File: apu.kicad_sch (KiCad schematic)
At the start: 0 parts

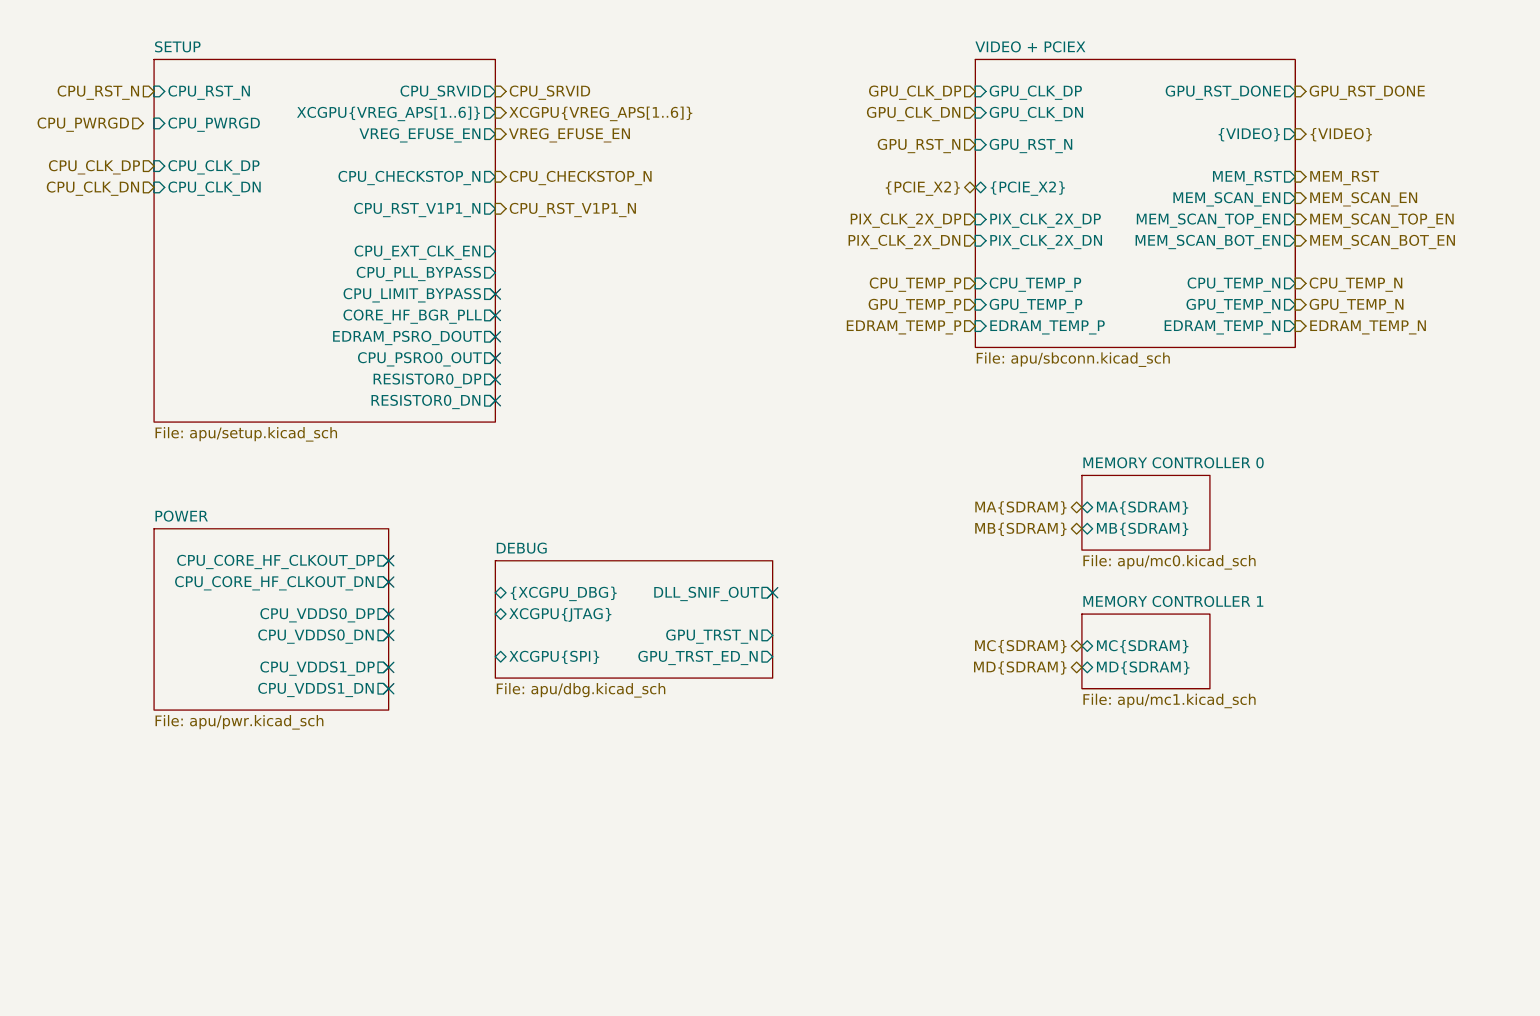
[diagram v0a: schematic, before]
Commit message: Cleanup & Debug I/O
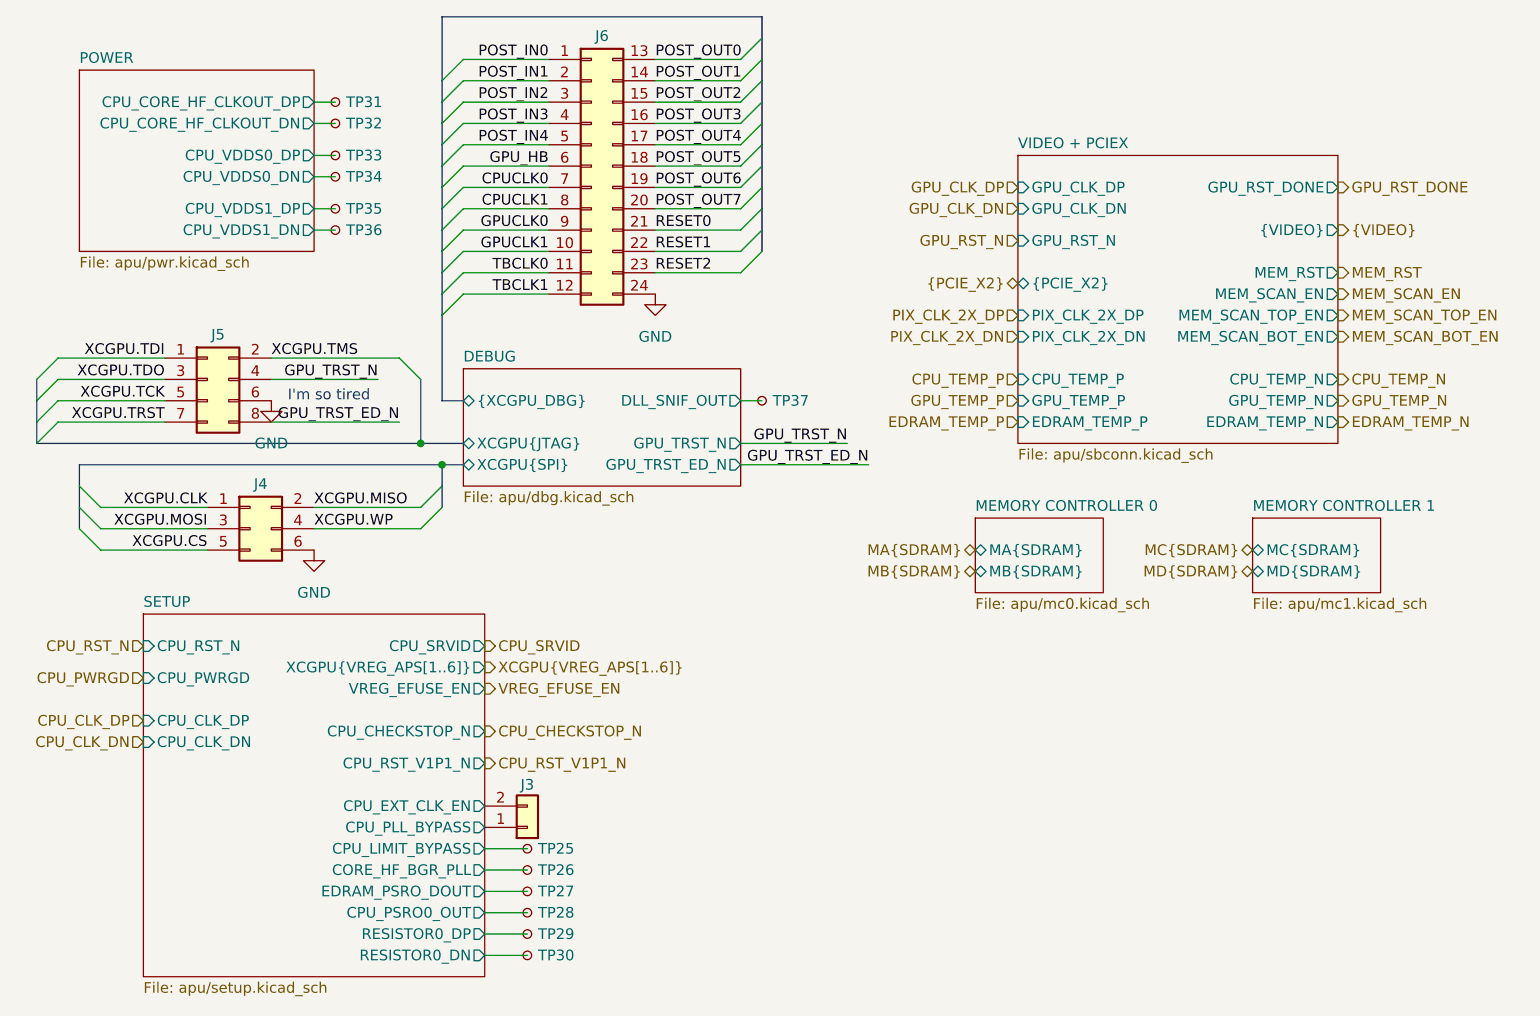
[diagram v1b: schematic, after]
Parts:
- added J3: Conn_01x02, symbol Connector_Generic:Conn_01x02
- added J4: Conn_02x03_Odd_Even, symbol Connector_Generic:Conn_02x03_Odd_Even
- added J5: Conn_02x04_Odd_Even, symbol Connector_Generic:Conn_02x04_Odd_Even
- added J6: Conn_02x12_Top_Bottom, symbol Connector_Generic:Conn_02x12_Top_Bottom
- added TP25, TP26, TP27, TP28, TP29, TP30, TP31, TP32, TP33, TP34, TP35, TP36, TP37: TestPoint_Small, symbol Connector:TestPoint_Small
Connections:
- net DEBUG/DLL_SNIF_OUT: now also TP37.1
- net POWER/CPU_CORE_HF_CLKOUT_DN: now also TP32.1
- net POWER/CPU_CORE_HF_CLKOUT_DP: now also TP31.1
- net POWER/CPU_VDDS0_DN: now also TP34.1
- net POWER/CPU_VDDS0_DP: now also TP33.1
- net POWER/CPU_VDDS1_DN: now also TP36.1
- net POWER/CPU_VDDS1_DP: now also TP35.1
- net SETUP/CORE_HF_BGR_PLL: now also TP26.1
- net SETUP/CPU_EXT_CLK_EN: now also J3.2 (Pin_2)
- net SETUP/CPU_LIMIT_BYPASS: now also TP25.1
- net SETUP/CPU_PLL_BYPASS: now also J3.1 (Pin_1)
- net SETUP/CPU_PSRO0_OUT: now also TP28.1
- net SETUP/EDRAM_PSRO_DOUT: now also TP27.1
- net SETUP/RESISTOR0_DN: now also TP30.1
- net SETUP/RESISTOR0_DP: now also TP29.1
- new net CPUCLK0: J6.7 (Pin_7)
- new net CPUCLK1: J6.8 (Pin_8)
- new net GND: J4.6 (Pin_6), J5.6 (Pin_6), J6.24 (Pin_24)
- new net GPUCLK0: J6.9 (Pin_9)
- new net GPUCLK1: J6.10 (Pin_10)
- new net GPU_HB: J6.6 (Pin_6)
- new net GPU_TRST_ED_N: J5.8 (Pin_8)
- new net GPU_TRST_N: J5.4 (Pin_4)
- new net POST_IN0: J6.1 (Pin_1)
- new net POST_IN1: J6.2 (Pin_2)
- new net POST_IN2: J6.3 (Pin_3)
- new net POST_IN3: J6.4 (Pin_4)
- new net POST_IN4: J6.5 (Pin_5)
- new net POST_OUT0: J6.13 (Pin_13)
- new net POST_OUT1: J6.14 (Pin_14)
- new net POST_OUT2: J6.15 (Pin_15)
- new net POST_OUT3: J6.16 (Pin_16)
- new net POST_OUT4: J6.17 (Pin_17)
- new net POST_OUT5: J6.18 (Pin_18)
- new net POST_OUT6: J6.19 (Pin_19)
- new net POST_OUT7: J6.20 (Pin_20)
- new net RESET0: J6.21 (Pin_21)
- new net RESET1: J6.22 (Pin_22)
- new net RESET2: J6.23 (Pin_23)
- new net TBCLK0: J6.11 (Pin_11)
- new net TBCLK1: J6.12 (Pin_12)
- new net XCGPU.CLK: J4.1 (Pin_1)
- new net XCGPU.CS: J4.5 (Pin_5)
- new net XCGPU.MISO: J4.2 (Pin_2)
- new net XCGPU.MOSI: J4.3 (Pin_3)
- new net XCGPU.TCK: J5.5 (Pin_5)
- new net XCGPU.TDI: J5.1 (Pin_1)
- new net XCGPU.TDO: J5.3 (Pin_3)
- new net XCGPU.TMS: J5.2 (Pin_2)
- new net XCGPU.TRST: J5.7 (Pin_7)
- new net XCGPU.WP: J4.4 (Pin_4)
- no-connect marks 13 -> 0
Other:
- note added: "I'm so tired"

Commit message: Debug Connectors
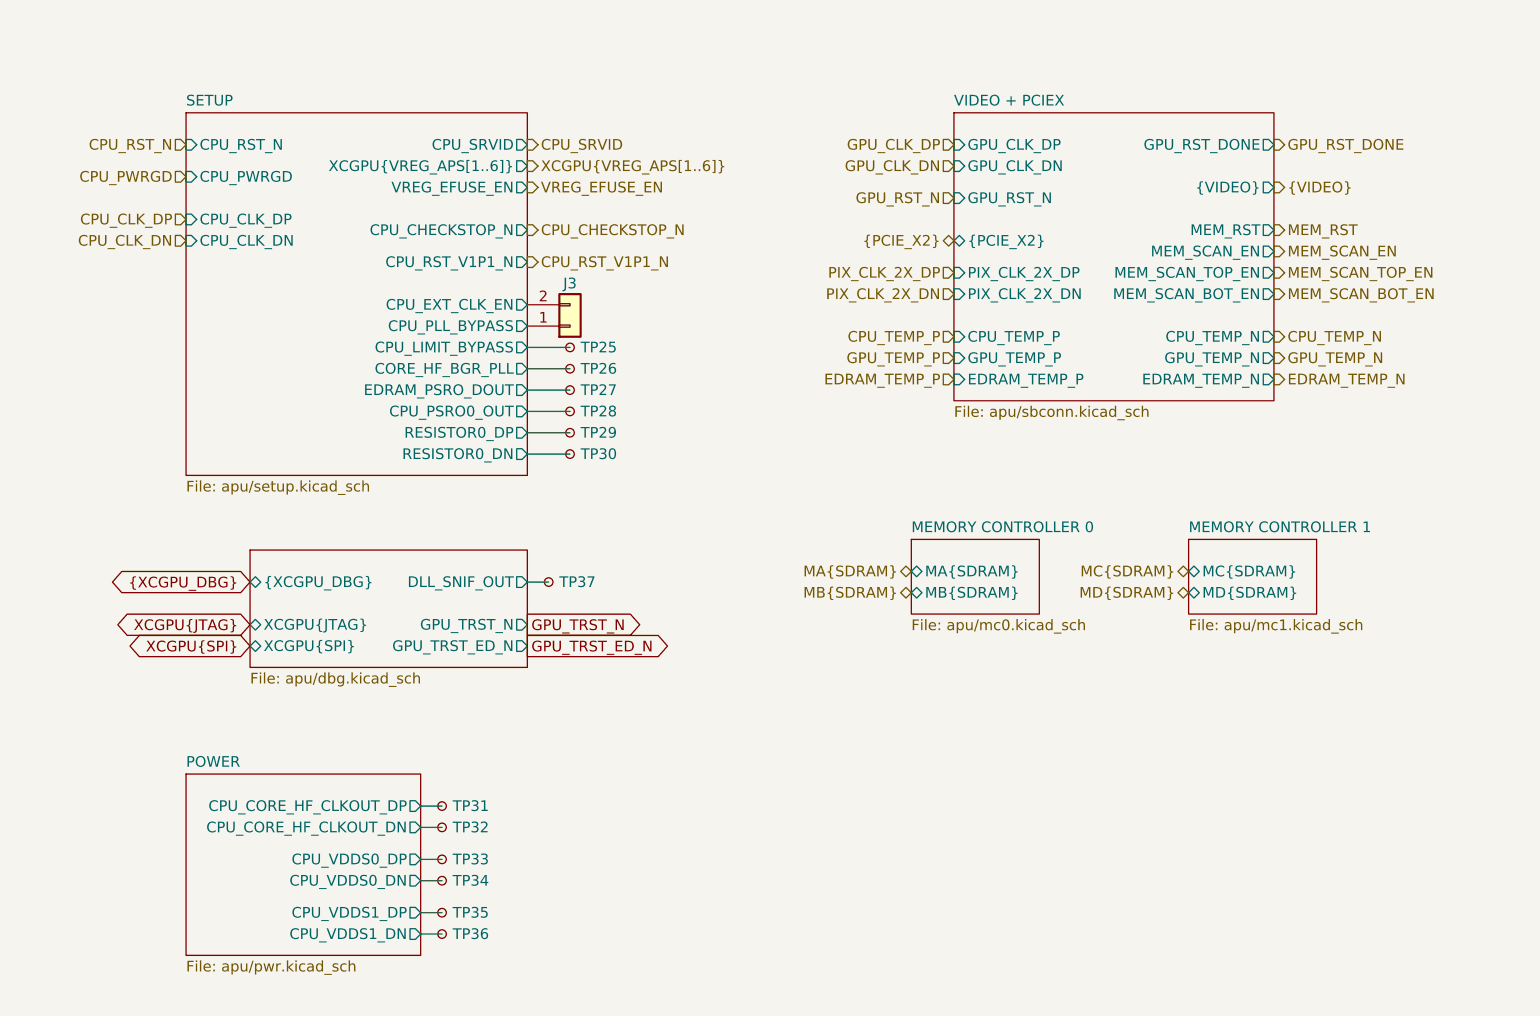
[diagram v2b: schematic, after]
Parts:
- removed J4: Conn_02x03_Odd_Even, symbol Connector_Generic:Conn_02x03_Odd_Even
- removed J5: Conn_02x04_Odd_Even, symbol Connector_Generic:Conn_02x04_Odd_Even
- removed J6: Conn_02x12_Top_Bottom, symbol Connector_Generic:Conn_02x12_Top_Bottom
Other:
- note removed: "I'm so tired"
- moved on the sheet: J3, TP25, TP26, TP27, TP28, TP29, TP30, TP31, TP32, TP33, TP34, TP35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
